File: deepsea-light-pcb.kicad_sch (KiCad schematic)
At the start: 8 parts, among them CN1 XT60PW-M, U1 Pico, U2 2604-1106, U3 2604-1106, U4 2604-1106, U5 2604-1106, U6 SparkFun_BabyBuck_5V, U7 SparkFun_RS485_Breakout

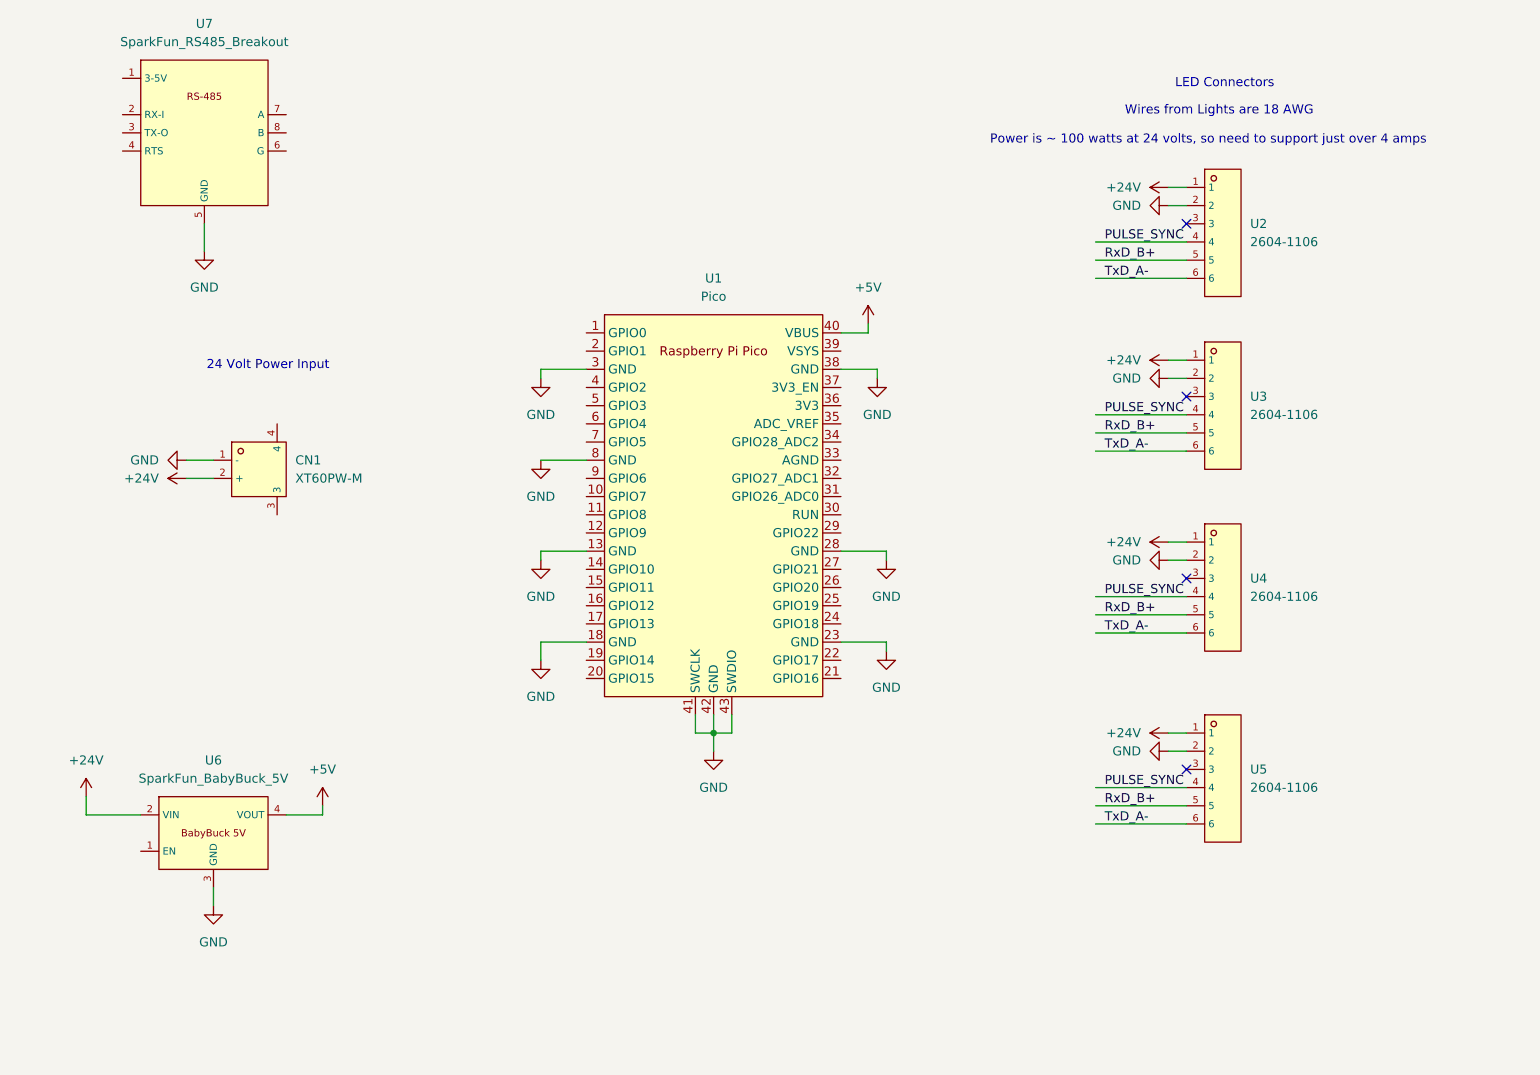
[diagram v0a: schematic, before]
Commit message: updates
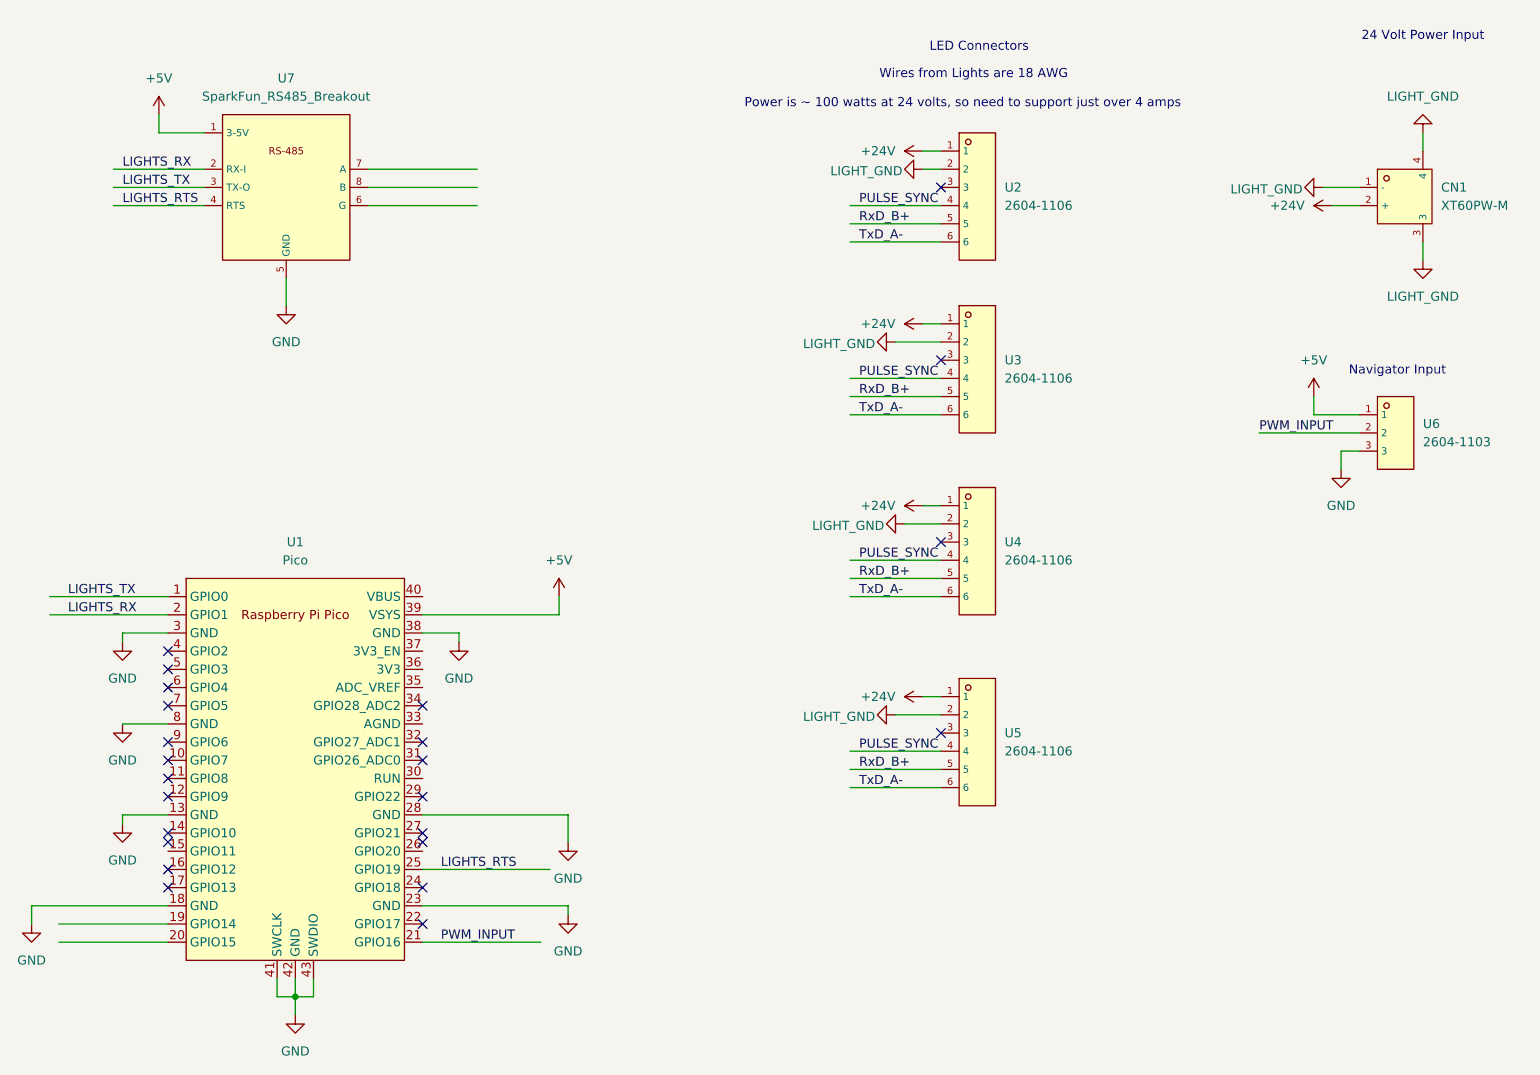
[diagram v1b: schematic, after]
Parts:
- removed U6: SparkFun_BabyBuck_5V, Deepsea_light_lib:SparkFun_BabyBuck_5V, symbol Deepsea_light_lib:SparkFun_BabyBuck_5V
- added U6: 2604-1103, Deepsea_light_lib:CONN-TH_2604-1103, symbol Deepsea_light_lib:2604-1103
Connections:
- net +5V: now also U1.39 (VSYS), U7.1 (3-5V), U6.1; no longer U1.40 (VBUS)
- net GND: now also U6.3; no longer CN1.1 (-), U2.2, U3.2, U4.2, U5.2
- net LIGHT_GND: now reaches CN1.3
- net LIGHT_GND: now also CN1.1 (-), CN1.4, U2.2, U3.2, U4.2, U5.2
- net LIGHTS_RX: now reaches U7.2 (RX-I)
- net LIGHTS_RX: now also U1.2 (GPIO1)
- net LIGHTS_TX: now reaches U7.3 (TX-O)
- net LIGHTS_TX: now also U1.1 (GPIO0)
- net LIGHTS_RTS: now reaches U7.4 (RTS)
- net LIGHTS_RTS: now also U1.25 (GPIO19)
- net PWM_INPUT: now reaches U1.21 (GPIO16)
- net PWM_INPUT: now also U6.2
- no-connect marks 4 -> 24
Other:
- note added: "Navigator Input"
- moved on the sheet: CN1, U1, U2, U3, U4, U5, U7
